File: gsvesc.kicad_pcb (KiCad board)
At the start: 4 copper layers, 111 x 111 mm, 113 parts, among them J1 Conn_01x06, J10 PHASE_C, J11 PHASE_A, J12 NTC, J13 PHASE_B, J14 Conn_02x04_Odd_Even, J2 Conn_01x06, J3 Conn_01x06, J4 Conn_01x05, J5 Conn_01x03, J6 USB_B_Mini, J7 BAT+, J8 BAT-, Q1 NVMFS5C604, Q2 NVMFS5C604, Q3 NVMFS5C604, Q4 NVMFS5C604, Q5 NVMFS5C604, Q6 NVMFS5C604, U1 STM32F405RGTx, U2 IRU1010-33, U3 DRV8301DCAR, U4 AD8418, U5 AD8418, U6 AD8418, Y1 ABM3B 8MHz

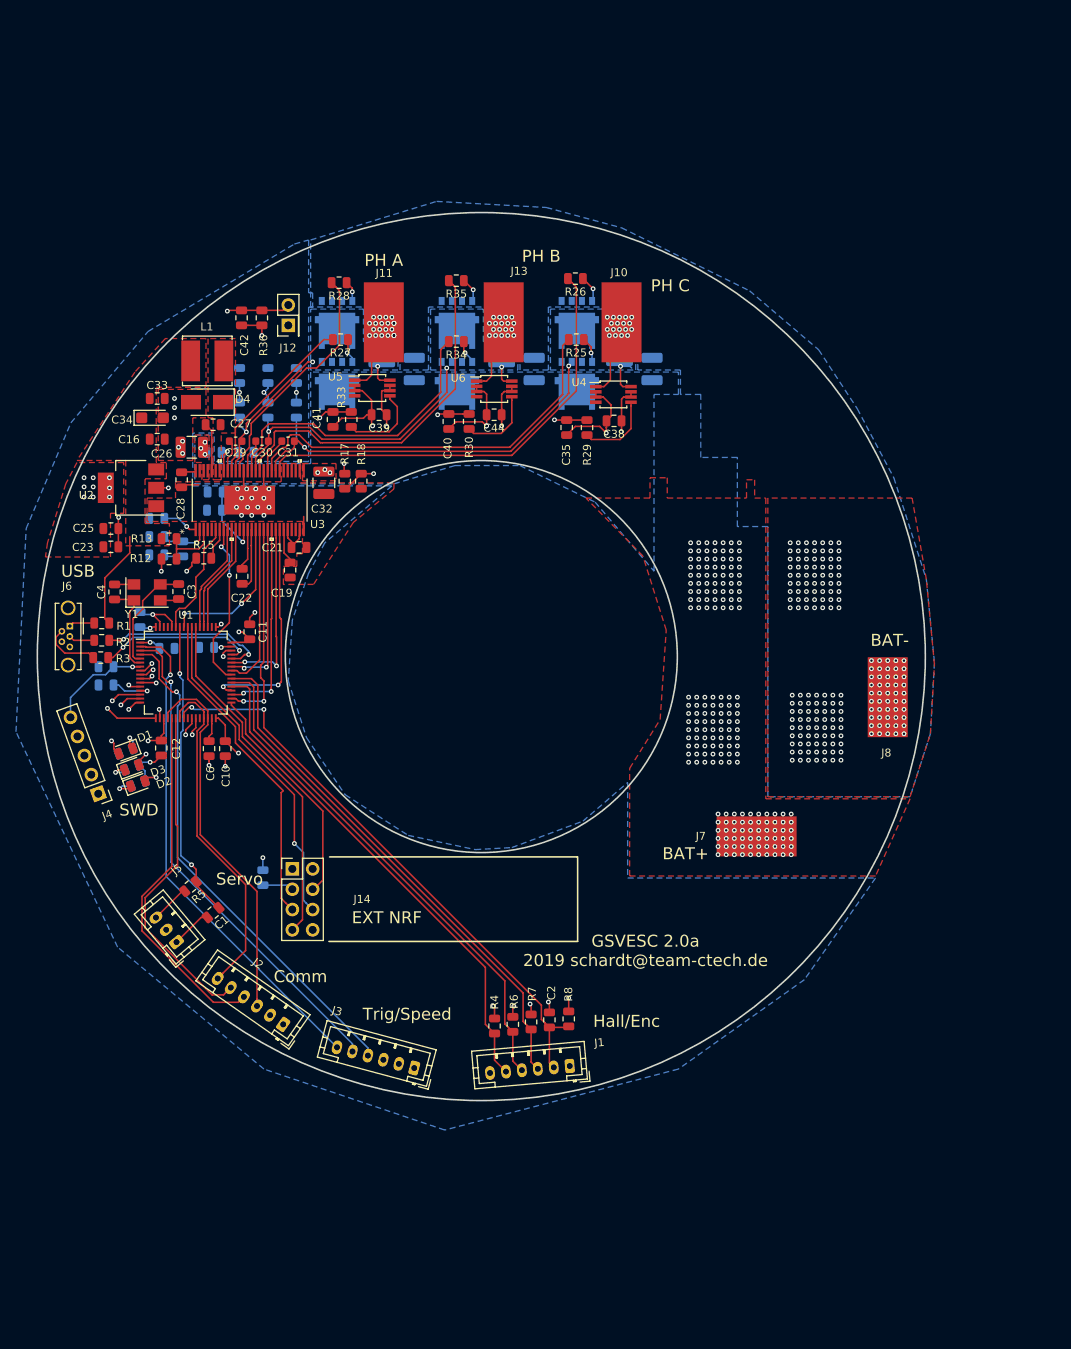
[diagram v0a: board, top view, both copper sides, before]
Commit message: gsesc v3, work in progress
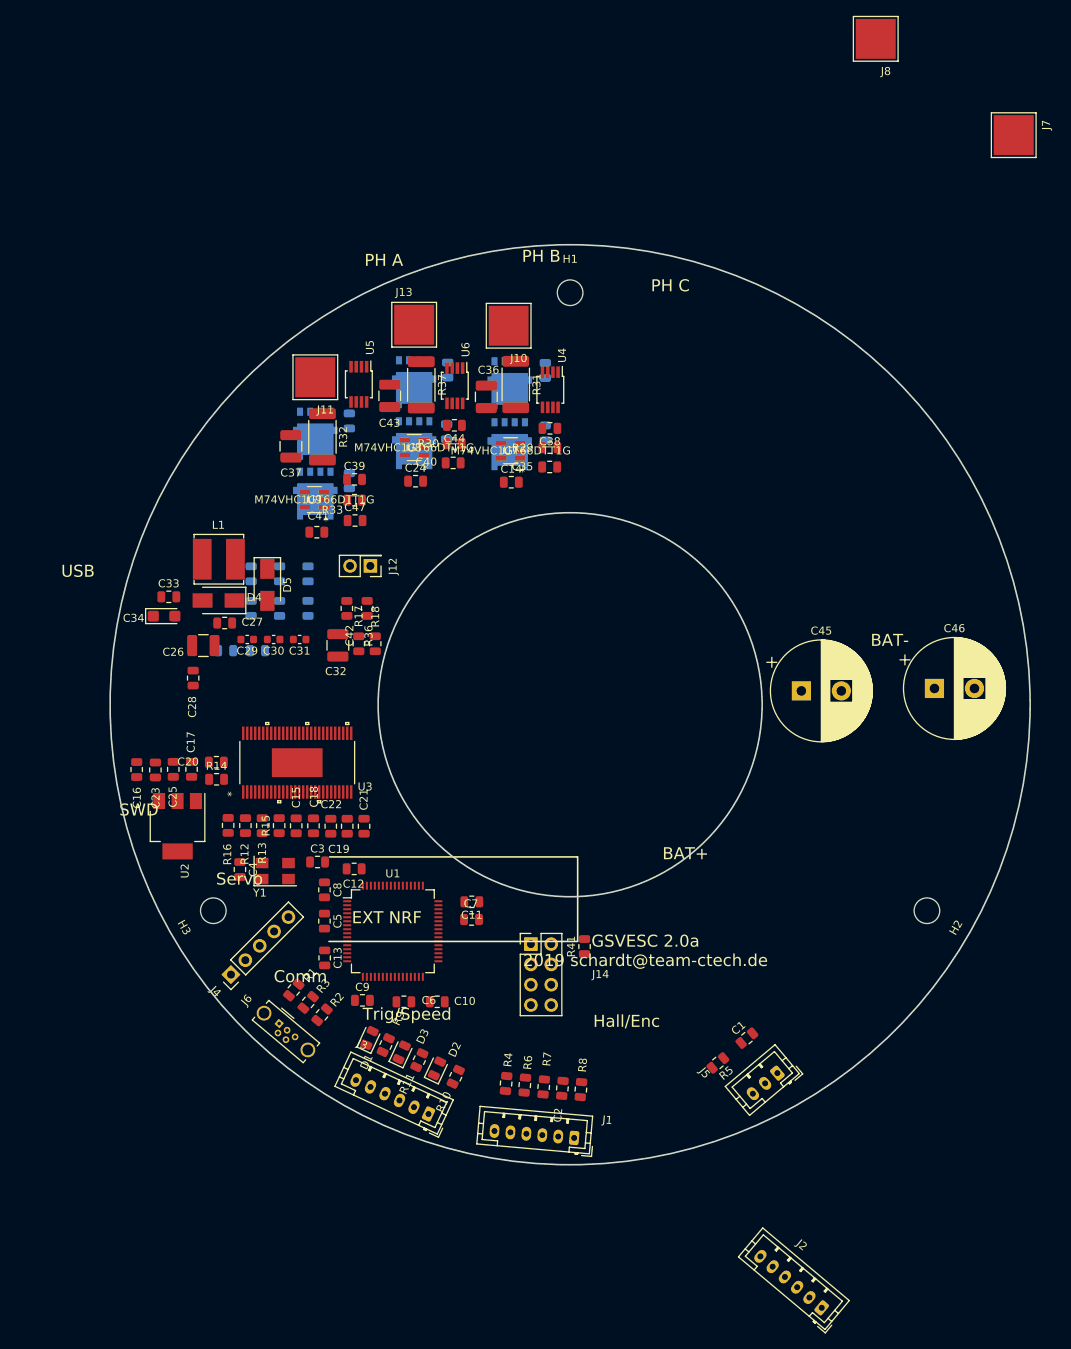
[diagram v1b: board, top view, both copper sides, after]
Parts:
- added C14: 1n00, Capacitor_SMD:C_0805_2012Metric, F.Cu at (92.6, 72.2)
- added C24: 1n00, Capacitor_SMD:C_0805_2012Metric, F.Cu at (80.7, 72.1)
- added C45: 680u/80V, Capacitor_THT:CP_Radial_D12.5mm_P5.00mm, F.Cu at (128.9, 98.3)
- added C46: 680u/80V, Capacitor_THT:CP_Radial_D12.5mm_P5.00mm, F.Cu at (145.5, 98.0)
- added C47: 1n00, Capacitor_SMD:C_0805_2012Metric, F.Cu at (73.1, 77.0)
- added D5: D, Diode_SMD:D_SMA, F.Cu at (62.2, 85.0)
- added H1: MountingHole, MountingHole:MountingHole_3.2mm_M3, F.Cu at (100.0, 48.5)
- added H2: MountingHole, MountingHole:MountingHole_3.2mm_M3, F.Cu at (144.6, 125.8)
- added H3: MountingHole, MountingHole:MountingHole_3.2mm_M3, F.Cu at (55.4, 125.8)
- added U7: M74VHC1GT66DTT1G, gsvesc:M74VHC1GT66DTT1G, F.Cu at (92.6, 68.2)
- added U8: M74VHC1GT66DTT1G, gsvesc:M74VHC1GT66DTT1G, F.Cu at (80.5, 67.9)
- added U9: M74VHC1GT66DTT1G, gsvesc:M74VHC1GT66DTT1G, F.Cu at (68.0, 74.4)
- C13, C15, C17, C18, C20, C5, C7, C8, C9, R10, R11, R14, R16, R31, R32, R37, R41, R9: moved to F.Cu
- C35, C40, C41: value 4n70 -> 1n00
- C36, C37, C43: value 47u0/100V -> 10u0/100V; moved to F.Cu
- J10, J11, J13, J7, J8: footprint Connector_Wire:SolderWirePad_1x01_SMD_5x10mm -> gsvesc:TestPoint_Pad_5.0x5.0mm
- R25, R26, R27, R28, R34, R35: moved to B.Cu
- R29, R30, R33: value 100R -> 1k00
- moved J7 93.4 mm to (155.4, 28.8)
- moved J8 82.3 mm to (138.2, 16.8)
- moved J5 76.9 mm to (125.9, 146.1), turned to 220 degrees
- moved J2 76.1 mm to (131.4, 175.4), turned to 140 degrees
- moved R5 69.5 mm to (118.5, 144.8)
- moved C1 68.5 mm to (122.1, 141.7), turned to 40 degrees
- moved J6 56.1 mm to (63.6, 139.9), turned to 320 degrees
- moved R2 54.3 mm to (69.0, 138.8), turned to 230 degrees
- moved R10 54.1 mm to (85.7, 146.5), turned to 65 degrees
- moved R1 51.8 mm to (65.5, 135.7), turned to 230 degrees
- moved D2 51.6 mm to (83.4, 145.5), turned to 65 degrees
- moved R11 51.3 mm to (81.2, 144.4), turned to 65 degrees
- moved C9 50.3 mm to (74.0, 137.0), turned to 0 degrees
- moved R3 50.3 mm to (67.3, 137.2), turned to 230 degrees
- moved R9 49.1 mm to (77.0, 142.5), turned to 65 degrees
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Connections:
- net /POWER_CTRL/SUPPLY renamed /DRV8301/VBAT
- C3 pad 2: Net-(C3-Pad2) -> GND
- C41 pad 1: /MCU/CURRENT_1 -> Net-(C41-Pad1)
- J14 pad 4: Net-(J14-Pad4) -> /NRF/GPIO1
- J14 pad 6: Net-(J14-Pad6) -> /NRF/GPIO2
- J14 pad 8: Net-(J14-Pad8) -> /NRF/GPIO3
- J3 pad 3: Net-(J3-Pad3) -> /MCU/PC5
- U1 pad 28: /MCU/PB2 -> /NRF/GPIO1
- U1 pad 54: /MCU/PD2 -> /POWER/CURR_FILTER
- U1 pad 55: /MCU/PB3 -> /NRF/GPIO2
- U1 pad 56: /MCU/PB4 -> /NRF/GPIO3
- U1 pad 6: GND -> Net-(C4-Pad2)
- Y1 pad 1: GND -> Net-(C4-Pad2)
- Y1 pad 2: Net-(C3-Pad2) -> GND
- Y1 pad 4: Net-(C4-Pad2) -> GND
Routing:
- net GND: track 96.5 -> 0.00 mm, vias 212 -> 0
- net /MCU/TEMP_MOTOR: track 73.3 -> 0.00 mm, vias 2 -> 0
- net /MCU/ADC_TEMP: track 70.7 -> 0.00 mm, vias 2 -> 0
- net /MCU/CURRENT_3: track 69.3 -> 0.00 mm, vias 2 -> 0
- net /MCU/HALL_3: track 66.1 -> 0.00 mm
- net /MCU/HALL_2: track 64.8 -> 0.00 mm
- net /MCU/HALL_1: track 63.5 -> 0.00 mm
- net /MCU/HALL_ROT_B: track 63.3 -> 0.00 mm, vias 1 -> 0
- net /MCU/HALL_ROT_A: track 62.5 -> 0.00 mm, vias 1 -> 0
- net /MCU/HALL_TRIG: track 62.2 -> 0.00 mm, vias 1 -> 0
- net VCC: track 57.0 -> 0.00 mm, vias 26 -> 0
- net /DRV8301/GL_C: track 56.3 -> 0.00 mm
- net /DRV8301/SH_C: track 56.1 -> 0.00 mm, vias 3 -> 0
- net /MCU/CURRENT_2: track 54.6 -> 0.00 mm, vias 2 -> 0
- net /DRV8301/SENS_C: track 53.8 -> 0.00 mm, vias 2 -> 0
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- removed copper zone on F.Cu, net +5V
- removed copper zone on B.Cu, net /DRV8301/SH_A
- removed copper zone on B.Cu, net /DRV8301/SH_B
- removed copper zone on B.Cu, net /DRV8301/SH_C
- removed copper zone on B.Cu, net /DRV8301/VBAT
- removed copper zone on F.Cu, net /DRV8301/VBAT
- removed copper zone on B.Cu, net /POWER/PHASE_A
- removed copper zone on B.Cu, net /POWER/PHASE_B
- removed copper zone on B.Cu, net /POWER/PHASE_C
- removed copper zone on B.Cu, net GND
- removed copper zone on F.Cu, net GND
- removed copper zone on In2.Cu, net GND
- removed copper zone on F.Cu, net Net-(C27-Pad1)
- removed copper zone on F.Cu, net VCC
- removed copper zone on In1.Cu, net VCC
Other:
- board size 111 x 111 mm -> 115 x 115 mm
- rule via_min_size: 0.4 -> 0.6
